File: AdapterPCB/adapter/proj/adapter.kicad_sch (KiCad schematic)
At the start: 36 parts, among them J2 VGA, U1 SN74LVC245APW, U2 SN74LVC245APW

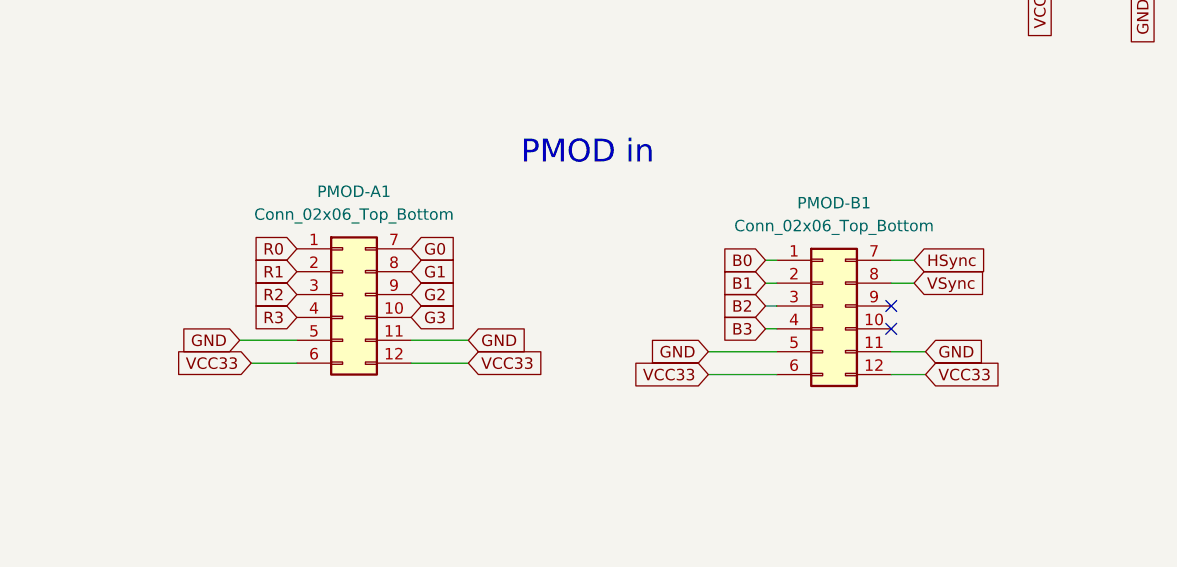
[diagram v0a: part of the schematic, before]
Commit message: fixed drc
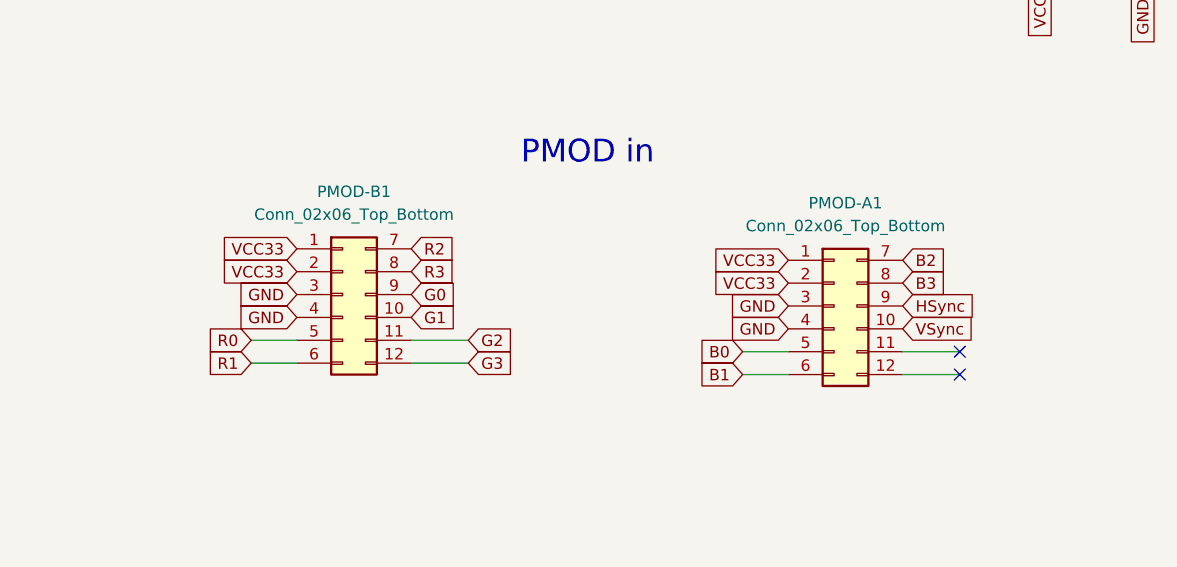
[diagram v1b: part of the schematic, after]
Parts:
- removed PMOD-B1: Conn_02x06_Top_Bottom, Connector_PinHeader_2.54mm:PinHeader_2x06_P2.54mm_Horizontal, symbol Connector_Generic:Conn_02x06_Top_Bottom
- added PMOD-A1: Conn_02x06_Top_Bottom, Connector_PinHeader_2.54mm:PinHeader_2x06_P2.54mm_Horizontal, symbol Connector_Generic:Conn_02x06_Top_Bottom
- U1, U2: footprint Package_SO:TSSOP-20_4.4x6.5mm_P0.65mm -> Package_SO:SOIC-20W_7.5x12.8mm_P1.27mm
- renumbered PMOD-A1 to PMOD-B1
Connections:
- net B0: now also PMOD-A1.5 (Pin_5)
- net B1: now also PMOD-A1.6 (Pin_6)
- net B2: now also PMOD-A1.7 (Pin_7)
- net B3: now also PMOD-A1.8 (Pin_8)
- net G0: now also PMOD-B1.9 (Pin_9); no longer PMOD-B1.7 (Pin_7)
- net G1: now also PMOD-B1.10 (Pin_10); no longer PMOD-B1.8 (Pin_8)
- net G2: now also PMOD-B1.11 (Pin_11); no longer PMOD-B1.9 (Pin_9)
- net G3: now also PMOD-B1.12 (Pin_12); no longer PMOD-B1.10 (Pin_10)
- net GND: now also PMOD-B1.3 (Pin_3), PMOD-B1.4 (Pin_4), PMOD-A1.3 (Pin_3), PMOD-A1.4 (Pin_4); no longer PMOD-B1.11 (Pin_11), PMOD-B1.5 (Pin_5)
- net HSync: now also PMOD-A1.9 (Pin_9)
- net R0: now also PMOD-B1.5 (Pin_5); no longer PMOD-B1.1 (Pin_1)
- net R1: now also PMOD-B1.6 (Pin_6); no longer PMOD-B1.2 (Pin_2)
- net R2: now also PMOD-B1.7 (Pin_7); no longer PMOD-B1.3 (Pin_3)
- net R3: now also PMOD-B1.8 (Pin_8); no longer PMOD-B1.4 (Pin_4)
- net VCC33: now also PMOD-B1.1 (Pin_1), PMOD-B1.2 (Pin_2), PMOD-A1.1 (Pin_1), PMOD-A1.2 (Pin_2); no longer PMOD-B1.12 (Pin_12), PMOD-B1.6 (Pin_6)
- net VSync: now also PMOD-A1.10 (Pin_10)
